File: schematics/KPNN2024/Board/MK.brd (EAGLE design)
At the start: 68.9 x 68.9 mm, 18 parts

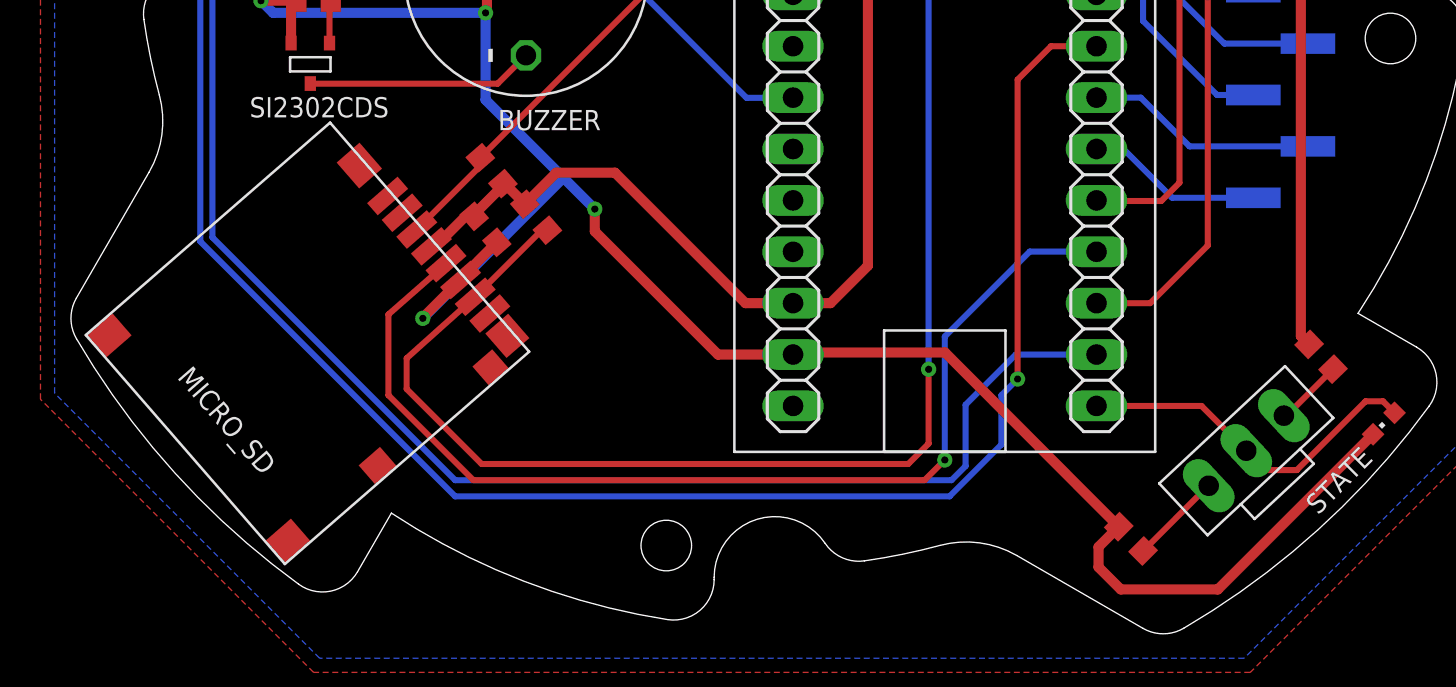
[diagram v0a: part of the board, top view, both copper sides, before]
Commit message: сдклвл платы а мботрен зз
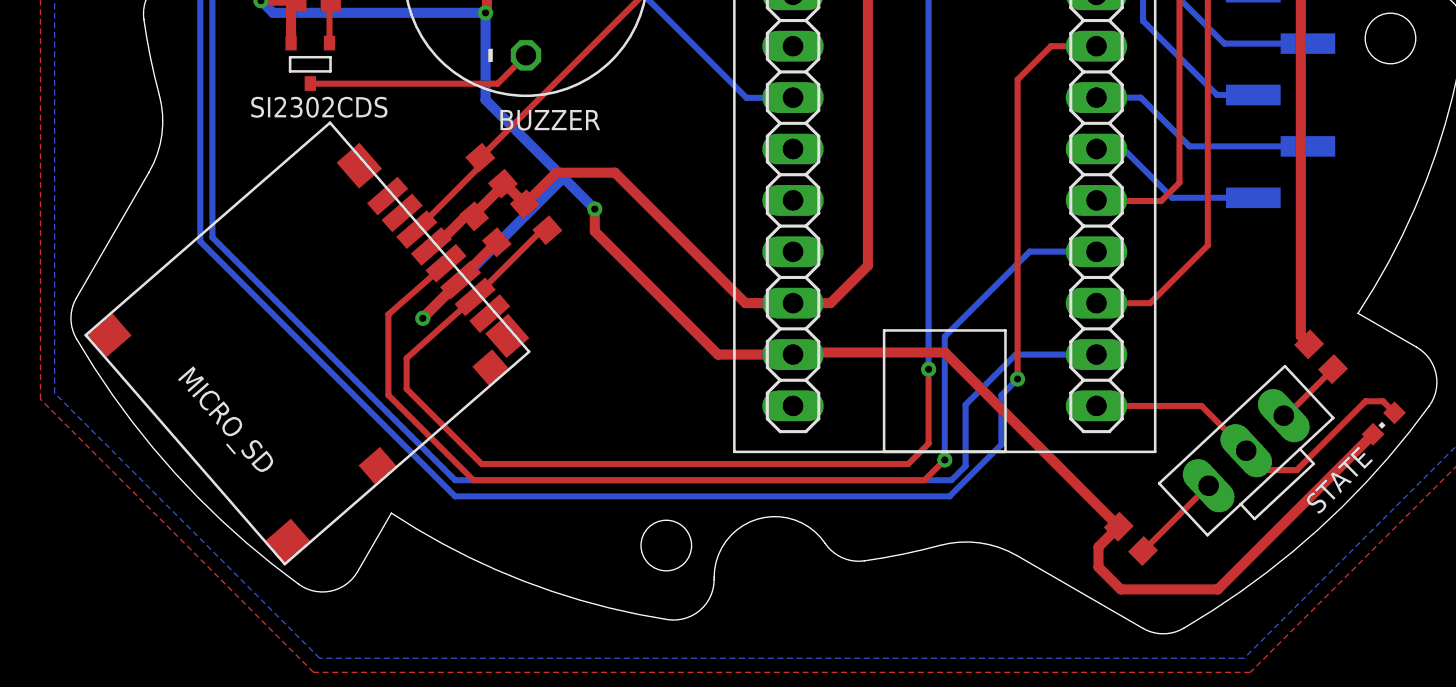
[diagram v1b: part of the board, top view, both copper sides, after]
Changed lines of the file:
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@@
 <?xml version="1.0" encoding="utf-8"?>
 <!DOCTYPE eagle SYSTEM "eagle.dtd">
-<eagle version="9.4.2">
+<eagle version="9.6.2">
 <drawing>
 <settings>
-<setting alwaysvectorfont="yes"/>
+<setting alwaysvectorfont="no"/>
 <setting verticaltext="up"/>
 </settings>
@@
 </autorouter>
 <elements>
-<element name="MICRO_SD" library="UNKNOWN-2024" package="SD" value="SD" x="16.7814875" y="9.654290625" smashed="yes" rot="R131">
-<attribute name="NAME" x="16.42138125" y="14.641296875" size="1" layer="25" font="vector" ratio="15" rot="R131"/>
+<element name="MICRO_SD" library="UNKNOWN-2024" package="SD" value="SD" x="16.78" y="9.65" smashed="yes" rot="R131">
+<attribute name="NAME" x="16.419890625" y="14.637003125" size="1" layer="25" font="vector" ratio="15" rot="R131"/>
 </element>
 <element name="BUZZER" library="CanCubeSat" package="BUZZER-S8R12" value="BUZZERS8R6" x="28.7" y="38.8" smashed="yes" rot="R90">
@@
 <attribute name="VALUE" x="20.065" y="39.295" size="1" layer="27" font="vector" ratio="15"/>
 </element>
-<element name="U$2" library="UNKNOWN-2024" package="SWITCH_MSS" value="SWITCH_MSS" x="64.303021875" y="15.257525" smashed="yes" rot="R223">
-<attribute name="VALUE" x="64.924134375" y="20.4779875" size="1" layer="27" font="vector" ratio="15" rot="R223"/>
+<element name="U$2" library="UNKNOWN-2024" package="SWITCH_MSS" value="SWITCH_MSS" x="64.3" y="15.257525" smashed="yes" rot="R223">
+<attribute name="VALUE" x="64.9211125" y="20.4779875" size="1" layer="27" font="vector" ratio="15" rot="R223"/>
 </element>
 <element name="R1" library="rcl" library_urn="urn:adsk.eagle:library:334" package="R0603" package3d_urn="urn:adsk.eagle:package:23555/3" value="2k" x="58.6" y="10.9" smashed="yes" rot="R135">
@@
 <wire x1="17.0876875" y1="37.4123125" x2="17" y2="37.5" width="0.5" layer="1"/>
 <wire x1="23.6" y1="21.8" x2="23.6" y2="21.82985" width="0.5" layer="1"/>
-<wire x1="25.468565625" y1="23.698415625" x2="23.6" y2="21.82985" width="0.5" layer="1"/>
+<wire x1="25.467078125" y1="23.694125" x2="23.6" y2="21.82985" width="0.5" layer="1"/>
 <via x="23.6" y="21.8" extent="1-16" drill="0.35"/>
 <polygon width="0.3" layer="16">
@@
 <vertex x="4.7" y="17.8"/>
 </polygon>
-<wire x1="25.468565625" y1="23.698415625" x2="25.468565625" y2="23.76648125" width="0.5" layer="1"/>
+<wire x1="25.467078125" y1="23.694125" x2="25.468565625" y2="23.76648125" width="0.5" layer="1"/>
 <wire x1="25.468565625" y1="23.76648125" x2="27.25765" y2="25.55849375" width="0.5" layer="1"/>
 <wire x1="56.9" y1="63.19" x2="58.91" y2="63.19" width="0.5" layer="16"/>
@@
 <wire x1="28.642346875" y1="27.441503125" x2="30.198909375" y2="29" width="0.5" layer="1"/>
 <wire x1="30.198909375" y1="29" x2="33.1" y2="29" width="0.5" layer="1"/>
-<wire x1="24.0252375" y1="25.358778125" x2="24.2252375" y2="25.358778125" width="0.5" layer="1"/>
+<wire x1="24.02375" y1="25.3544875" x2="24.2252375" y2="25.358778125" width="0.5" layer="1"/>
 <wire x1="28.59895625" y1="27.501040625" x2="28.642346875" y2="27.441503125" width="0.5" layer="1"/>
 <wire x1="24.2252375" y1="25.358778125" x2="25.7079625" y2="26.841503125" width="0.5" layer="1"/>
@@
 <wire x1="34.487915625" y1="37.79" x2="41.9" y2="37.79" width="0.3" layer="1"/>
 <wire x1="26.442346875" y1="29.741503125" x2="34.487915625" y2="37.79" width="0.3" layer="1"/>
-<wire x1="23.303571875" y1="26.188959375" x2="26.39895625" y2="29.28434375" width="0.3" layer="1"/>
+<wire x1="23.302084375" y1="26.18466875" x2="26.39895625" y2="29.28434375" width="0.3" layer="1"/>
 <wire x1="26.39895625" y1="29.28434375" x2="26.442346875" y2="29.741503125" width="0.3" layer="1"/>
 </signal>
@@
 <contactref element="MICRO_SD" pad="CLK"/>
 <contactref element="STM" pad="24"/>
-<wire x1="24.746903125" y1="24.528596875" x2="24.431915625" y2="24.213609375" width="0.3" layer="1"/>
+<wire x1="24.745415625" y1="24.52430625" x2="24.431915625" y2="24.213609375" width="0.3" layer="1"/>
 <wire x1="24.431915625" y1="24.213609375" x2="21.9" y2="21.9923625" width="0.3" layer="1"/>
 <wire x1="21.9" y1="21.9923625" x2="21.9" y2="18" width="0.3" layer="1"/>
@@
 <contactref element="STM" pad="35"/>
 <contactref element="MICRO_SD" pad="DAT0"/>
-<wire x1="26.19023125" y1="22.8682375" x2="26.12951875" y2="22.807525" width="0.3" layer="1"/>
+<wire x1="26.18874375" y1="22.863946875" x2="26.12951875" y2="22.807525" width="0.3" layer="1"/>
 <wire x1="26.12951875" y1="22.807525" x2="22.8" y2="19.824575" width="0.3" layer="1"/>
 <wire x1="22.8" y1="19.824575" x2="22.8" y2="18.3071125" width="0.3" layer="1"/>
@@
 <contactref element="R5" pad="2"/>
 <wire x1="29.75765" y1="26.15849375" x2="29.52099375" y2="26.199" width="0.3" layer="1"/>
-<wire x1="29.52099375" y1="26.199" x2="26.19023125" y2="22.8682375" width="0.3" layer="1"/>
+<wire x1="29.52099375" y1="26.199" x2="26.18874375" y2="22.863946875" width="0.3" layer="1"/>
 </signal>
 <signal name="SWITCH">
@@
 <contactref element="STM" pad="21"/>
 <contactref element="STATE" pad="A"/>
-<wire x1="64.303021875" y1="15.257525" x2="65.260546875" y2="14.3" width="0.3" layer="1"/>
+<wire x1="64.3" y1="15.257525" x2="65.260546875" y2="14.3" width="0.3" layer="1"/>
 <wire x1="65.260546875" y1="14.3" x2="66.8" y2="14.3" width="0.3" layer="1"/>
 <wire x1="71.06065625" y1="17.7" x2="71.630328125" y2="17.130328125" width="0.3" layer="1"/>
 <wire x1="66.8" y1="14.3" x2="70.2" y2="17.7" width="0.3" layer="1"/>
 <wire x1="70.2" y1="17.7" x2="71.06065625" y2="17.7" width="0.3" layer="1"/>
-<wire x1="64.303021875" y1="15.257525" x2="62.090546875" y2="17.47" width="0.3" layer="1"/>
+<wire x1="64.3" y1="15.257525" x2="62.090546875" y2="17.47" width="0.3" layer="1"/>
 <wire x1="62.090546875" y1="17.47" x2="56.9" y2="17.47" width="0.3" layer="1"/>
 </signal>
@@
 <contactref element="R1" pad="1"/>
 <contactref element="U$2" pad="3"/>
-<wire x1="62.44538125" y1="13.525246875" x2="62.4270875" y2="13.525246875" width="0.3" layer="1"/>
+<wire x1="62.442359375" y1="13.525246875" x2="62.4270875" y2="13.525246875" width="0.3" layer="1"/>
 <wire x1="62.4270875" y1="13.525246875" x2="59.201040625" y2="10.29895625" width="0.3" layer="1"/>
 </signal>
@@
 <contactref element="R2" pad="1"/>
 <contactref element="U$2" pad="1"/>
-<wire x1="66.160659375" y1="16.9898" x2="66.2917" y2="16.9898" width="0.3" layer="1"/>
+<wire x1="66.1576375" y1="16.9898" x2="66.2917" y2="16.9898" width="0.3" layer="1"/>
 <wire x1="68.590459375" y1="19.288559375" x2="66.2917" y2="16.9898" width="0.3" layer="1"/>
 </signal>
